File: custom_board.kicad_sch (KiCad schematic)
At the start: 18 parts, among them IC1 TMPM46BF10FG

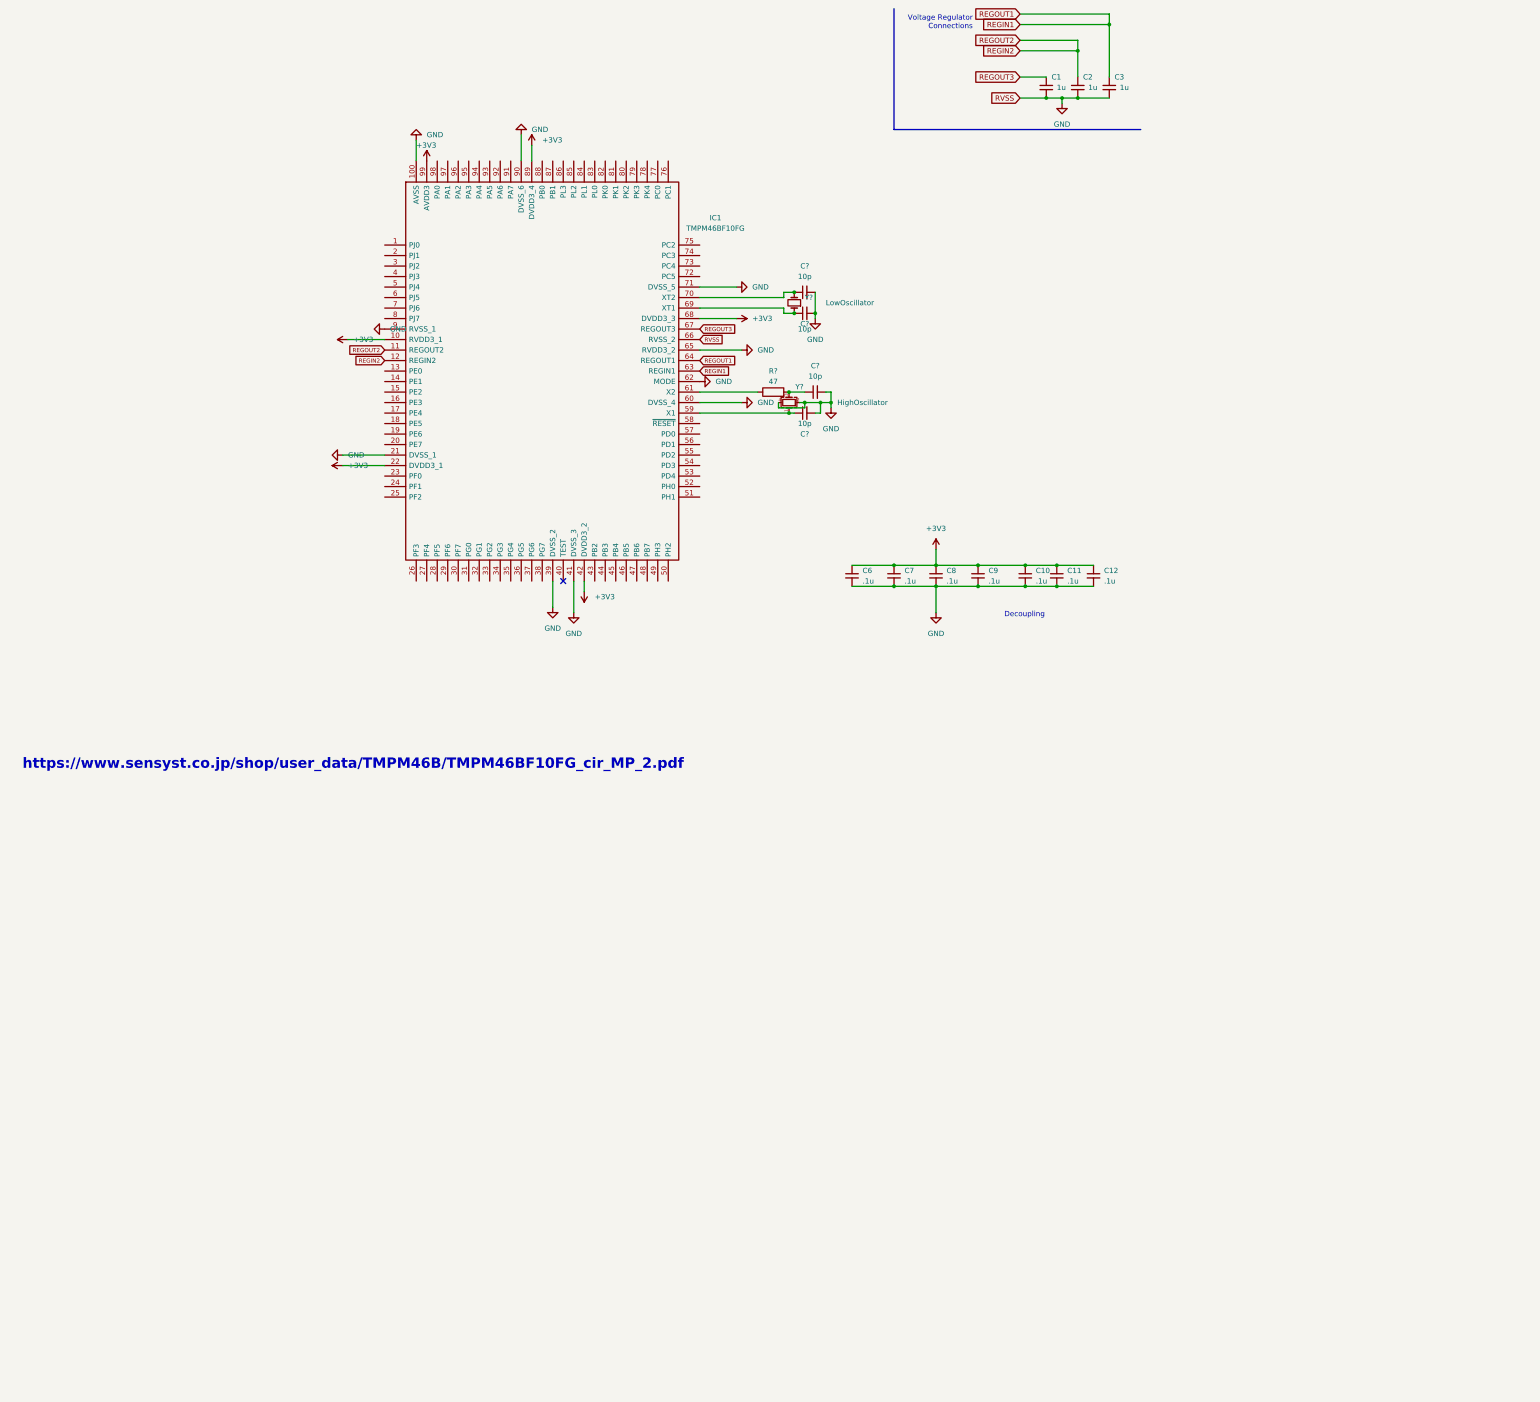
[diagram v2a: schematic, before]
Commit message: Working on hardware interfaces
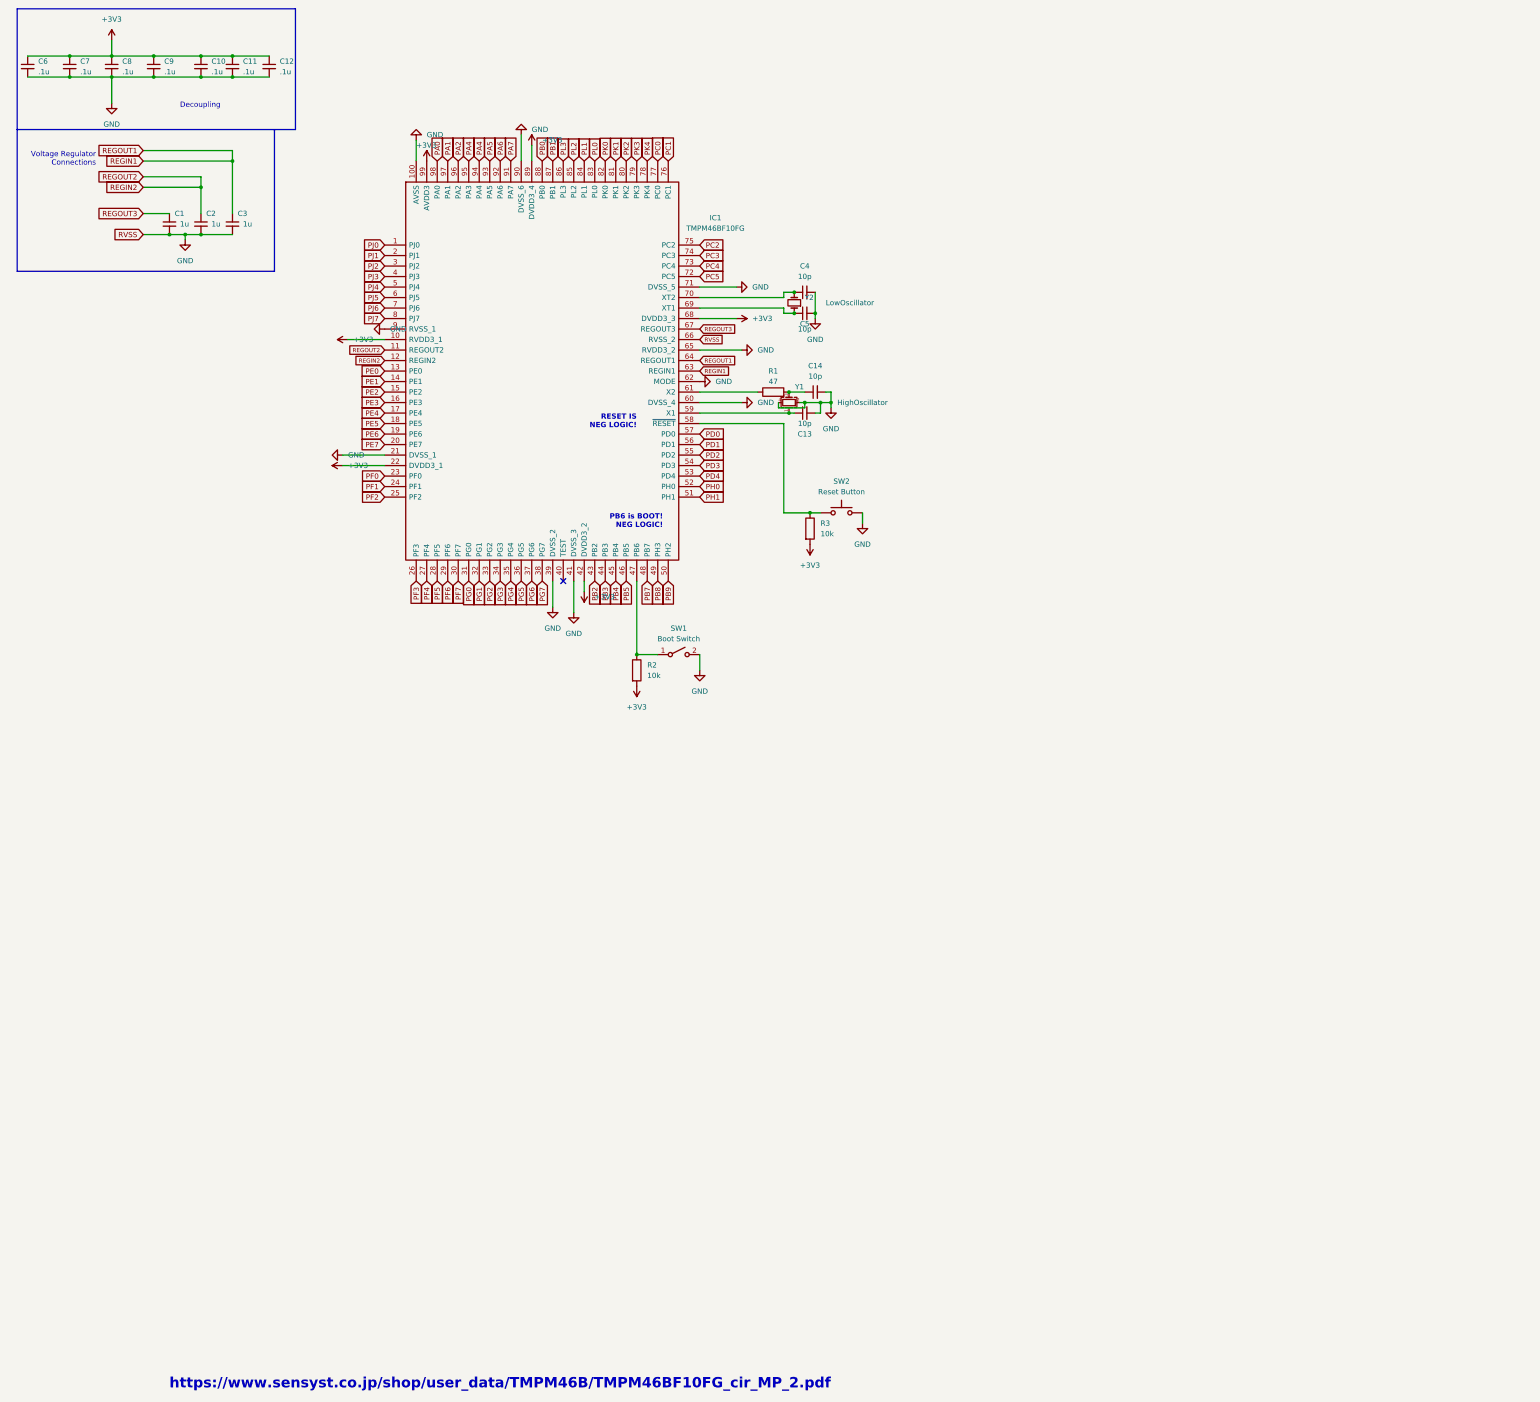
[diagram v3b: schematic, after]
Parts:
- added R2, R3: 10k, symbol Device:R
- added SW1: Boot Switch, symbol Switch:SW_SPST
- added SW2: Reset Button, symbol Switch:SW_Push
- gave numbers to parts that had none: 7
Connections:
- net +3V3: now also R2.2, R3.2
- net GND: now also SW1.2 (B), SW2.2
- net PJ0: now reaches IC1.1 (PJ0)
- net PE0: now reaches IC1.13 (PE0)
- net PE1: now reaches IC1.14 (PE1)
- net PE2: now reaches IC1.15 (PE2)
- net PE3: now reaches IC1.16 (PE3)
- net PE4: now reaches IC1.17 (PE4)
- net PE5: now reaches IC1.18 (PE5)
- net PE6: now reaches IC1.19 (PE6)
- net PJ1: now reaches IC1.2 (PJ1)
- net PE7: now reaches IC1.20 (PE7)
- net PF0: now reaches IC1.23 (PF0)
- net PF1: now reaches IC1.24 (PF1)
- net PF2: now reaches IC1.25 (PF2)
- net PF3: now reaches IC1.26 (PF3)
- net PF4: now reaches IC1.27 (PF4)
- net PF5: now reaches IC1.28 (PF5)
- net PF6: now reaches IC1.29 (PF6)
- net PJ2: now reaches IC1.3 (PJ2)
- net PF7: now reaches IC1.30 (PF7)
- net PG0: now reaches IC1.31 (PG0)
- net PG1: now reaches IC1.32 (PG1)
- net PG2: now reaches IC1.33 (PG2)
- net PG3: now reaches IC1.34 (PG3)
- net PG4: now reaches IC1.35 (PG4)
- net PG5: now reaches IC1.36 (PG5)
- net PG6: now reaches IC1.37 (PG6)
- net PG7: now reaches IC1.38 (PG7)
- net PJ3: now reaches IC1.4 (PJ3)
- net PB2: now reaches IC1.43 (PB2)
- net PB3: now reaches IC1.44 (PB3)
- net PB4: now reaches IC1.45 (PB4)
- net PB5: now reaches IC1.46 (PB5)
- net at IC1.47 (PB6): now also R2.1, SW1.1 (A)
- net PB7: now reaches IC1.48 (PB7)
- net PB8: now reaches IC1.49 (PH3)
- net PJ4: now reaches IC1.5 (PJ4)
- net PB9: now reaches IC1.50 (PH2)
- net PH1: now reaches IC1.51 (PH1)
- net PH0: now reaches IC1.52 (PH0)
- net PD4: now reaches IC1.53 (PD4)
- net PD3: now reaches IC1.54 (PD3)
- net PD2: now reaches IC1.55 (PD2)
- net PD1: now reaches IC1.56 (PD1)
- net PD0: now reaches IC1.57 (PD0)
- net at IC1.58 (~{RESET}): now also R3.1, SW2.1
- net PJ5: now reaches IC1.6 (PJ5)
- net PJ6: now reaches IC1.7 (PJ6)
- net PC5: now reaches IC1.72 (PC5)
- net PC4: now reaches IC1.73 (PC4)
- net PC3: now reaches IC1.74 (PC3)
- net PC2: now reaches IC1.75 (PC2)
- net PC1: now reaches IC1.76 (PC1)
- net PC0: now reaches IC1.77 (PC0)
- net PK4: now reaches IC1.78 (PK4)
- net PK3: now reaches IC1.79 (PK3)
- net PJ7: now reaches IC1.8 (PJ7)
- net PK2: now reaches IC1.80 (PK2)
- net PK1: now reaches IC1.81 (PK1)
- net PK0: now reaches IC1.82 (PK0)
- net PL0: now reaches IC1.83 (PL0)
- net PL1: now reaches IC1.84 (PL1)
- net PL2: now reaches IC1.85 (PL2)
- net PL3: now reaches IC1.86 (PL3)
- net PB1: now reaches IC1.87 (PB1)
- net PB0: now reaches IC1.88 (PB0)
- net PA7: now reaches IC1.91 (PA7)
- net PA6: now reaches IC1.92 (PA6)
- net PA5: now reaches IC1.93 (PA5)
- net PA4: now reaches IC1.94 (PA4)
- net PA4: now also IC1.95 (PA3)
- net PA2: now reaches IC1.96 (PA2)
- net PA1: now reaches IC1.97 (PA1)
- net PA0: now reaches IC1.98 (PA0)
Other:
- note added: "PB6 is BOOT! NEG LOGIC!"
- note added: "RESET IS NEG LOGIC!"
- title: (none) -> Toshiba UC Board Schematic
- moved on the sheet: C1, C10, C11, C12, C2, C3, C6, C7, C8, C9

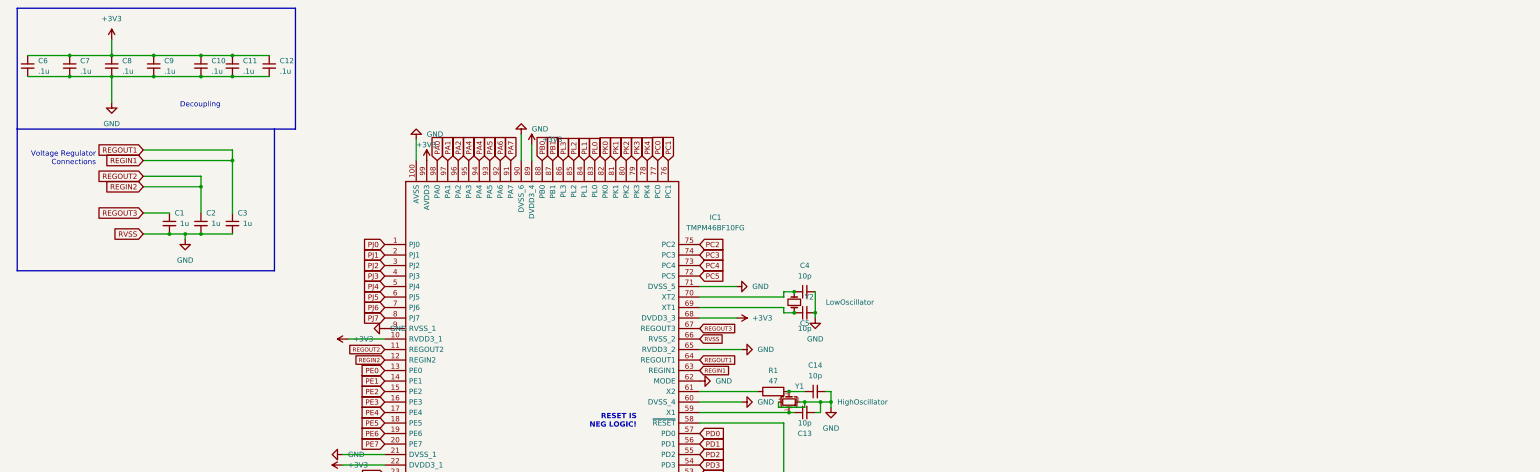
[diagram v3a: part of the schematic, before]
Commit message: Update custom_board.kicad_sch
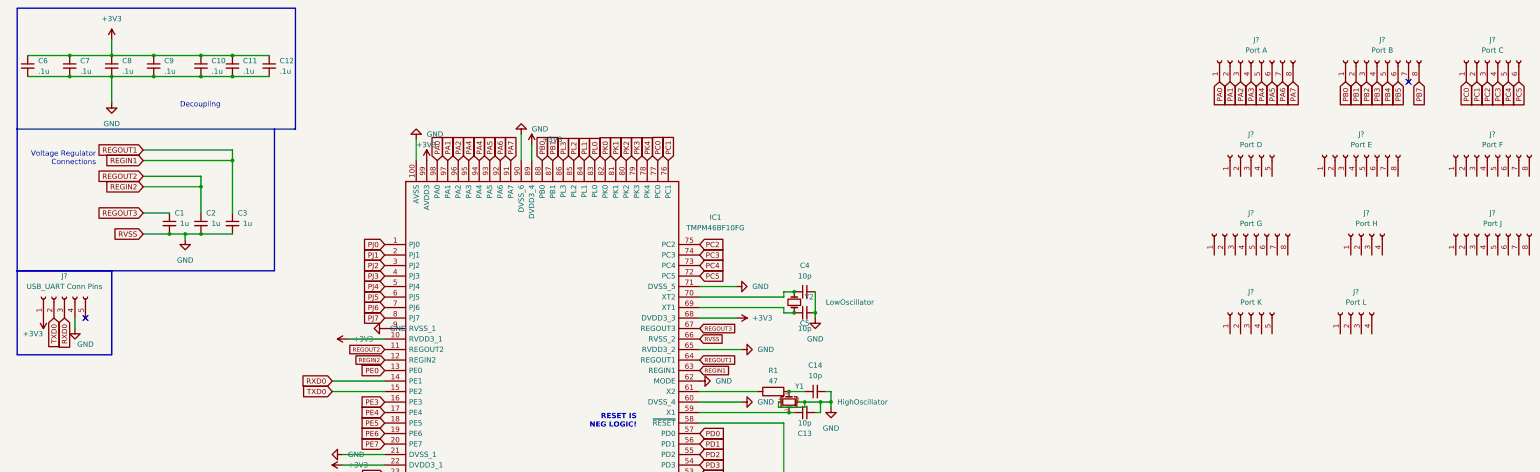
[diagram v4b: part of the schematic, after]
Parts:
- added J?: Port K, symbol Connector:Conn_01x05_Female
- added J?: Port E, symbol Connector:Conn_01x08_Female
- added J?: Port F, symbol Connector:Conn_01x08_Female
- added J?: Port L, symbol Connector:Conn_01x04_Female
- added J?: Port J, symbol Connector:Conn_01x08_Female
- added J?: Port H, symbol Connector:Conn_01x04_Female
- added J?: USB_UART Conn Pins, symbol Connector:Conn_01x05_Female
- added J?: Port A, symbol Connector:Conn_01x08_Female
- added J?: Port G, symbol Connector:Conn_01x08_Female
- added J?: Port B, symbol Connector:Conn_01x08_Female
- added J?: Port C, symbol Connector:Conn_01x06_Female
- added J?: Port D, symbol Connector:Conn_01x05_Female
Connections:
- net +3V3: now also J?.1 (Pin_1)
- net GND: now also J?.4 (Pin_4)
- net PA0: now also J?.1 (Pin_1)
- net PA1: now also J?.2 (Pin_2)
- net PA2: now also J?.3 (Pin_3)
- net PA4: now also J?.5 (Pin_5)
- net PA5: now also J?.6 (Pin_6)
- net PA6: now also J?.7 (Pin_7)
- net PA7: now also J?.8 (Pin_8)
- net PB0: now also J?.1 (Pin_1)
- net PB1: now also J?.2 (Pin_2)
- net PB2: now also J?.3 (Pin_3)
- net PB3: now also J?.4 (Pin_4)
- net PB4: now also J?.5 (Pin_5)
- net PB5: now also J?.6 (Pin_6)
- net PB7: now also J?.8 (Pin_8)
- net PC0: now also J?.1 (Pin_1)
- net PC1: now also J?.2 (Pin_2)
- net PC2: now also J?.3 (Pin_3)
- net PC3: now also J?.4 (Pin_4)
- net PC4: now also J?.5 (Pin_5)
- net PC5: now also J?.6 (Pin_6)
- net PE1 renamed RXD0
- net RXD0: now also J?.3 (Pin_3)
- net PE2 renamed TXD0
- net TXD0: now also J?.2 (Pin_2)
- new net PA3: J?.4 (Pin_4)
- no-connect marks 1 -> 3
